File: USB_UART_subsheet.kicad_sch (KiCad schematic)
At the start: 9 parts, among them U2 FT232RL

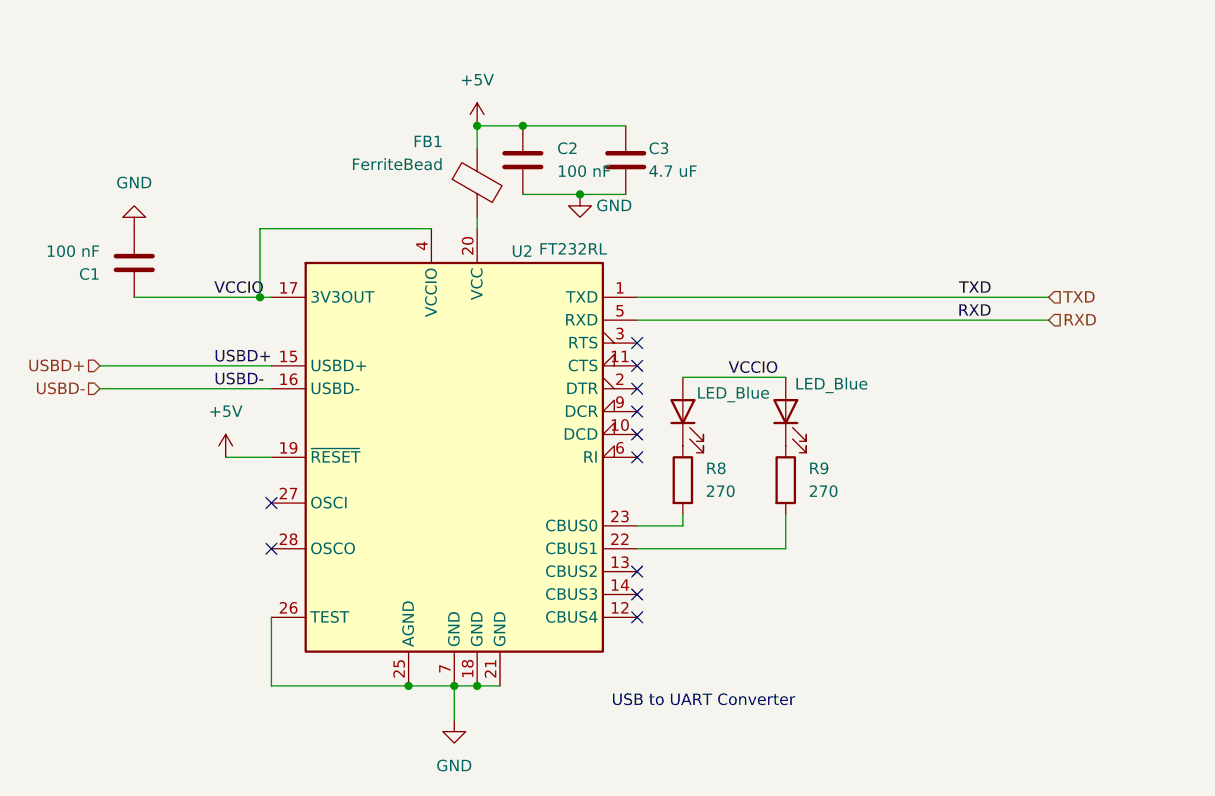
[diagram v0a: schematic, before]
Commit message: done
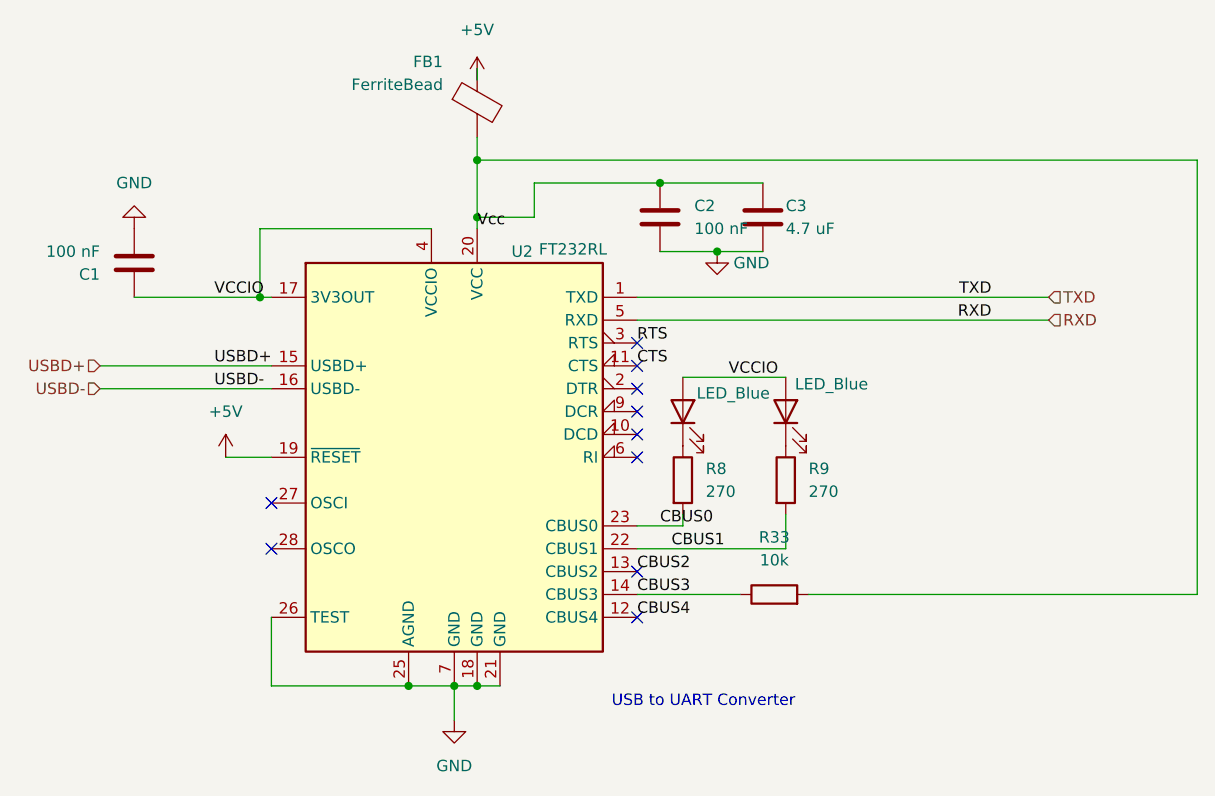
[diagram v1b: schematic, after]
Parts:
- added R33: 10k, Resistor_SMD:R_0805_2012Metric_Pad1.20x1.40mm_HandSolder, symbol Device:R
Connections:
- net +5V: no longer C2.1, C3.1
- net CBUS0 : now reaches R8.2, U2.23 (CBUS0)
- net CBUS1: now reaches R9.2, U2.22 (CBUS1)
- net CTS: now reaches U2.11 (CTS)
- net CBUS4: now reaches U2.12 (CBUS4)
- net CBUS2: now reaches U2.13 (CBUS2)
- net CBUS3: now reaches U2.14 (CBUS3)
- net CBUS3: now also R33.1
- net Vcc: now reaches FB1.2, U2.20 (VCC)
- net Vcc: now also C2.1, C3.1, R33.2
- net RTS: now reaches U2.3 (RTS)
- no-connect marks 11 -> 10
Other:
- moved on the sheet: C2, C3, FB1
